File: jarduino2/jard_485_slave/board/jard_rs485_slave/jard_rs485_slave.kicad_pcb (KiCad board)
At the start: 2 copper layers, 90 x 68 mm, 38 parts, among them J1 NETWORK IN, J2 NETWORK OUT, J3 ICSP, J4 LED, J5 Niveau bas, J6 Electrovanne 12V, J7 Niveau Haut, Q1 TIP41C, SW1 SW_Push, U1 LT1785xN8, U2 ATmega168-20PU, Y1 16MHz

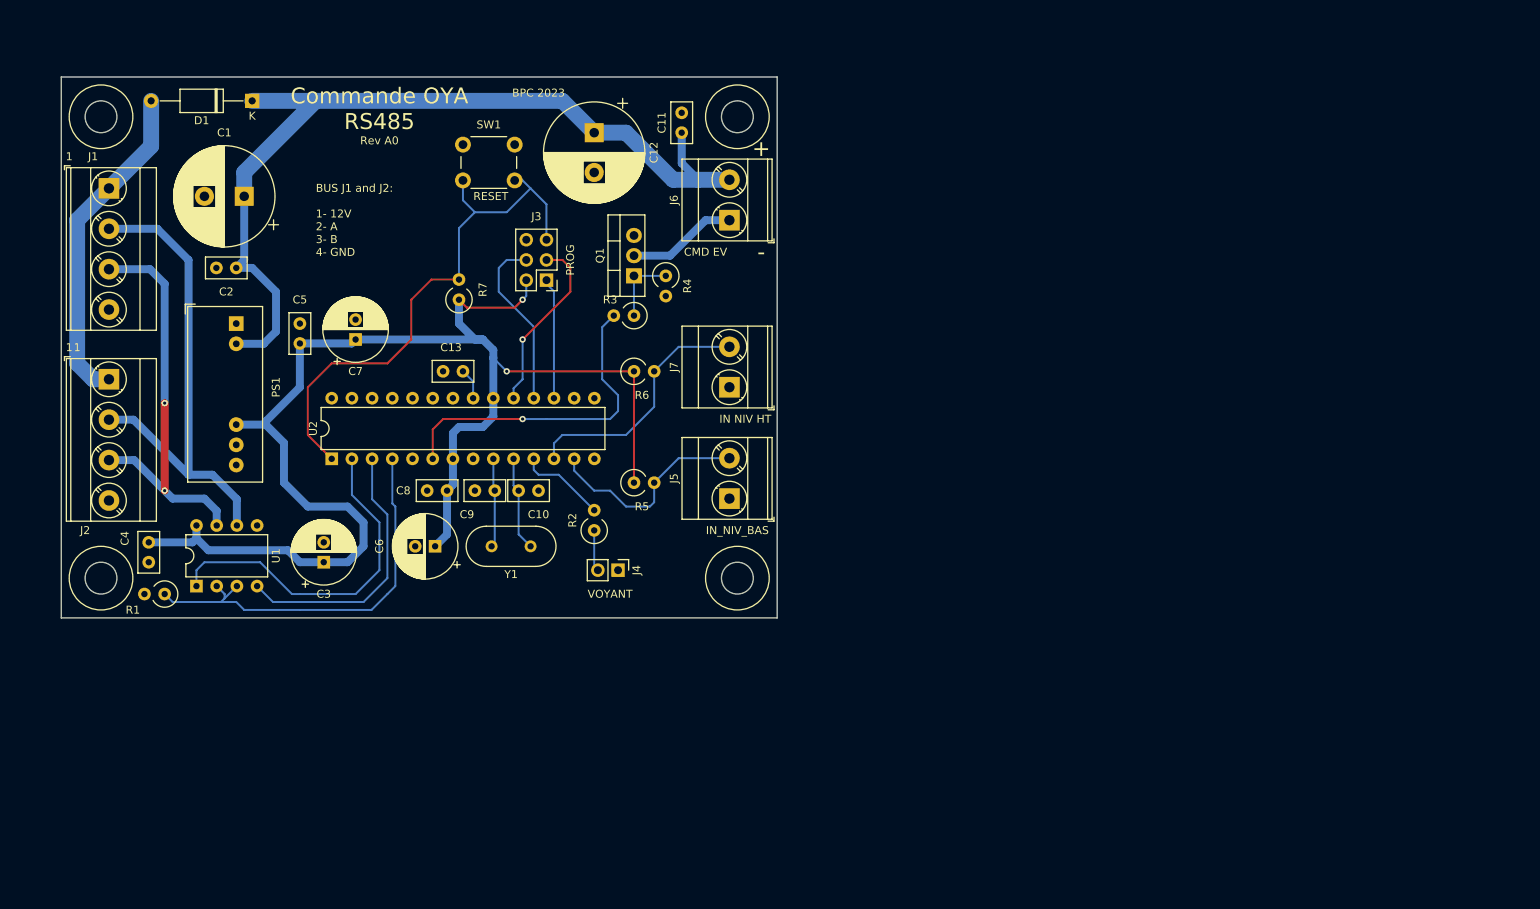
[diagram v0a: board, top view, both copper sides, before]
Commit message: ?
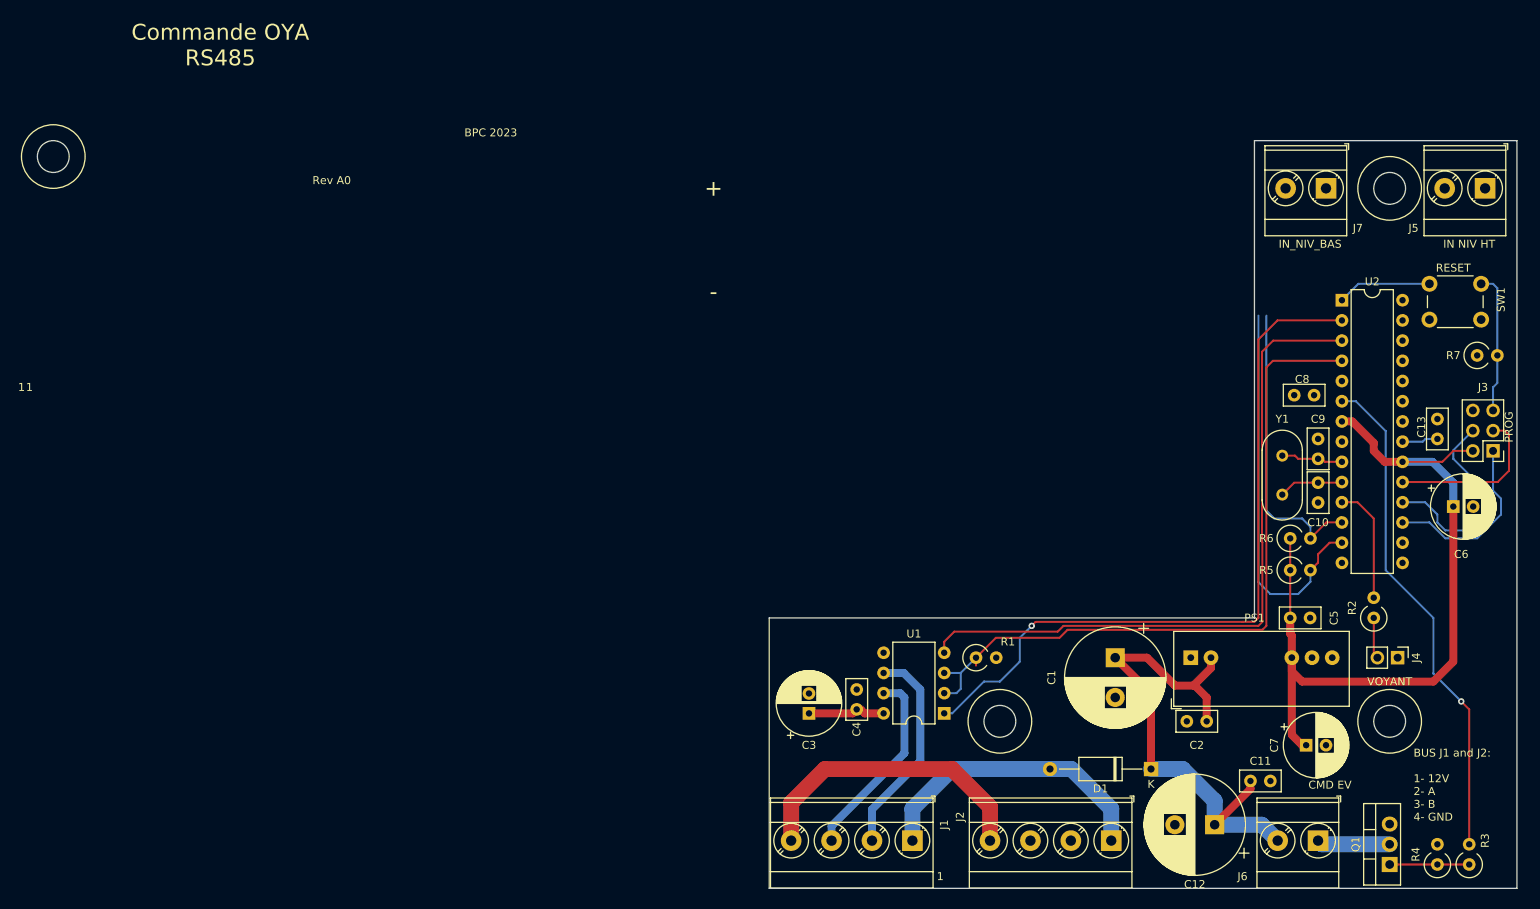
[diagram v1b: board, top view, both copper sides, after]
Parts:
- moved REF** 163.0 mm to (247.0, 125.0), turned to 90 degrees
- moved D1 140.8 mm to (217.0, 131.0)
- moved J2 138.7 mm to (212.0, 140.0), turned to 180 degrees
- moved C2 134.7 mm to (224.0, 125.0)
- moved C5 132.3 mm to (237.0, 112.0), turned to 180 degrees
- moved J1 130.1 mm to (187.0, 140.0), turned to 180 degrees
- moved C7 129.9 mm to (236.5, 128.0), turned to 0 degrees
- moved U2 128.6 mm to (241.0, 72.1), turned to 0 degrees
- moved R7 128.2 mm to (258.0, 79.0), turned to 0 degrees
- moved C6 128.1 mm to (255.0, 98.0), turned to 0 degrees
- moved PS1 127.1 mm to (222.0, 117.0), turned to 90 degrees
- moved R3 125.6 mm to (257.0, 143.0), turned to 90 degrees
- moved C13 125.1 mm to (253.0, 87.0), turned to 270 degrees
- moved C1 123.9 mm to (212.5, 117.0), turned to 270 degrees
- moved R4 122.0 mm to (253.0, 143.0), turned to 90 degrees
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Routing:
- net Vcc: track 175.1 -> 110.2 mm, vias 2 -> 0
- net TX: track 34.2 -> 87.0 mm
- net RX: track 43.7 -> 92.7 mm, vias 0 -> 1
- net Net-(C1-Pad1): track 112.9 -> 65.6 mm
- net RESET: track 69.6 -> 29.7 mm
- net TXEN: track 52.0 -> 90.6 mm
- net Net-(C1-Pad2): track 0.00 -> 37.7 mm
- net Net-(J1-Pad2): track 62.1 -> 27.0 mm
- net Net-(J1-Pad3): track 51.8 -> 24.6 mm, vias 2 -> 0
- net CMD_EV: track 41.4 -> 63.4 mm
- net IN_LVL_LOW: track 26.8 -> 48.8 mm
- net MISO: track 15.2 -> 22.9 mm
- net MOSI: track 22.1 -> 27.9 mm
- net IN_LVL_HIGH: track 31.6 -> 37.1 mm
- net Net-(J6-Pad1): track 13.8 -> 9.19 mm
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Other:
- board size 90 x 68 mm -> 94 x 94 mm
